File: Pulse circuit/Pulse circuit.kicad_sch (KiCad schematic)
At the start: 4 parts, among them U1 ESP32-DevKitC, U2 module_max30102, U3 module_max30102

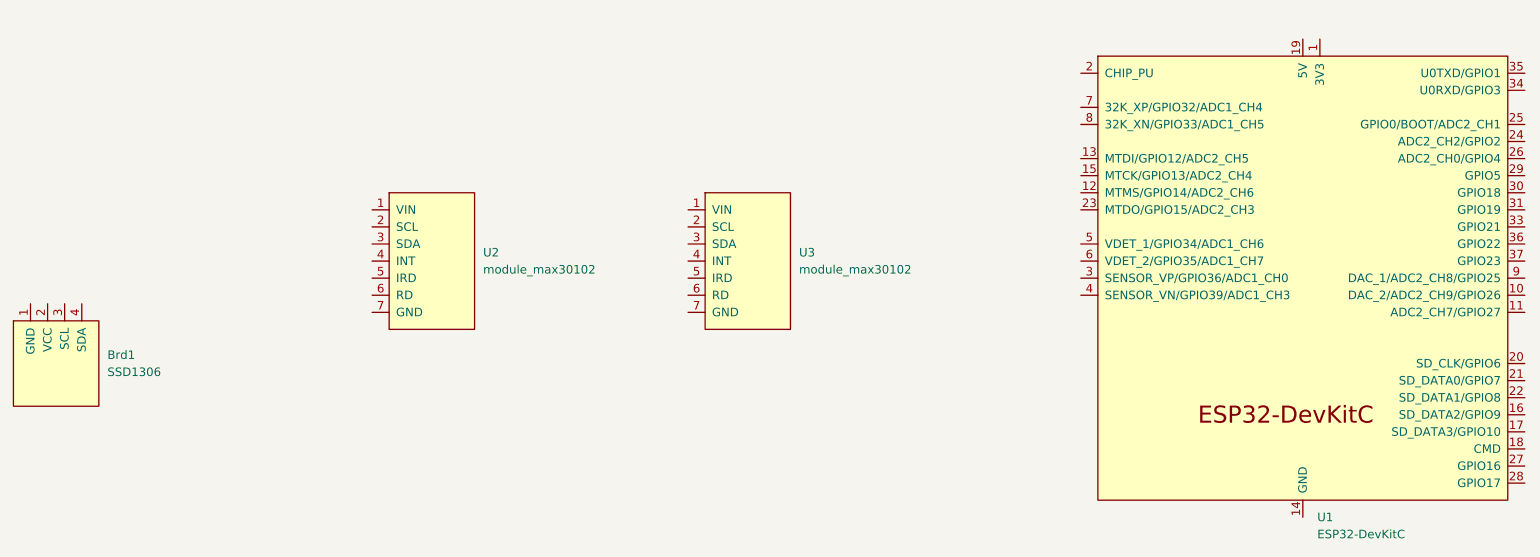
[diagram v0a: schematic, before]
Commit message: Updated with relative path
🎯
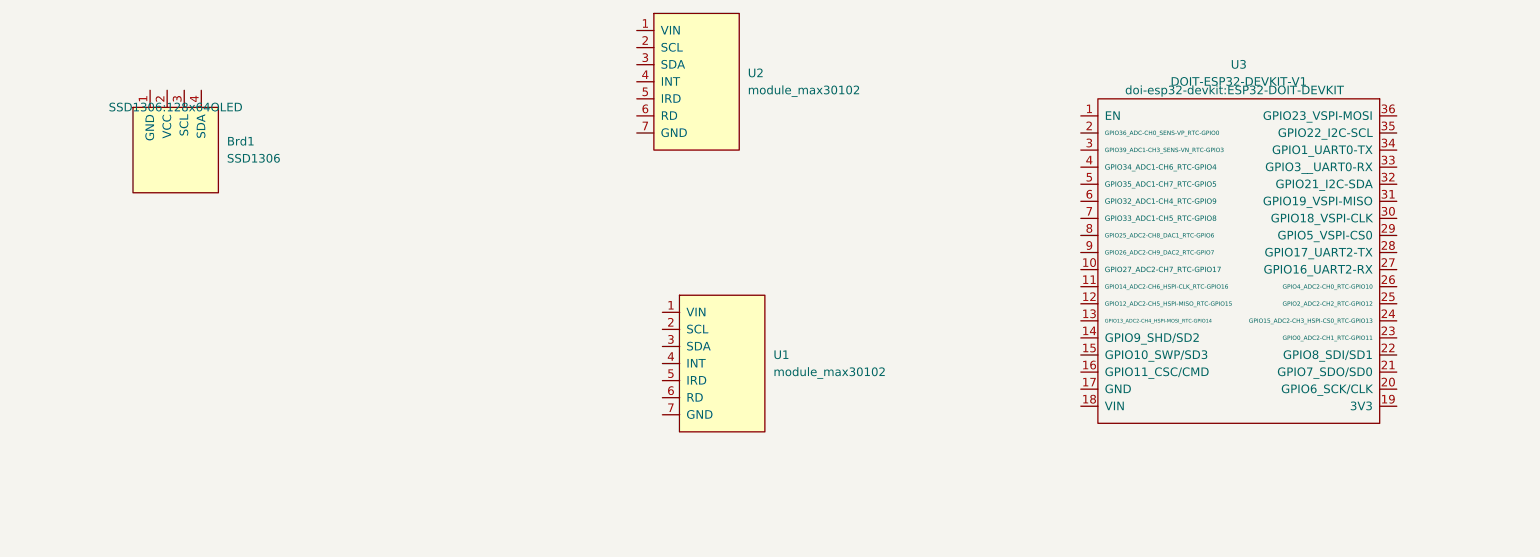
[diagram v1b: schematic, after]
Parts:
- removed U1: ESP32-DevKitC, PCM_Espressif:ESP32-DevKitC, symbol Espressif:ESP32-DevKitC
- removed U3: module_max30102, usini_sensors:module_max30102, symbol usini_sensors:module_max30102
- added U1: module_max30102, usini_sensors:module_max30102, symbol usini_sensors:module_max30102
- added U3: DOIT-ESP32-DEVKIT-V1, doi-esp32-devkit:ESP32-DOIT-DEVKIT, symbol doit-esp32-devkit-v1:DOIT-ESP32-DEVKIT-V1
